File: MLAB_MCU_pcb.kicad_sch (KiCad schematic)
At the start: 0 parts

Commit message: Collecting components and starting work on schematic
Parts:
- added C1, C2, C3, C4: 1u, Capacitor_SMD:C_0805_2012Metric_Pad1.18x1.45mm_HandSolder, symbol Device:C
- added J1, J2: Conn_01x02_Pin, Connector_PinHeader_2.54mm:PinHeader_1x02_P2.54mm_Vertical, symbol Connector:Conn_01x02_Pin
- added J3: Input Header, Connector_PinHeader_2.54mm:PinHeader_1x02_P2.54mm_Vertical, symbol Connector:Conn_01x02_Pin
- added J4: TBC05-02-1-G-G, TerminalBlock_Phoenix:TerminalBlock_Phoenix_MPT-0,5-2-2.54_1x02_P2.54mm_Horizontal, symbol Connector:Screw_Terminal_01x02
- added U1: TPS7A2012PDBVRG4, Package_TO_SOT_SMD:SOT-23-5, symbol Regulator_Linear:TPS7A20xxxDBV
- added U2: TPS7A2033PDBVR, Package_TO_SOT_SMD:SOT-23-5, symbol Regulator_Linear:TPS7A20xxxDBV
- added U3: DSC1101DL5-020.0000, 1_mlab_mcu_fp:VDFN6_2P5X2_MCH, symbol 1_mlab_mcu:DSC1101DL5-020.0000
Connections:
- new net: C2.1, J1.2 (Pin_2), U1.5 (OUT)
- new net: C1.1, J3.1 (Pin_1), J4.2 (Pin_2), U1.1 (IN), U1.3 (EN)
- new net: C3.1, J3.2 (Pin_2), J4.1 (Pin_1), U2.1 (IN), U2.3 (EN)
- new net: C4.1, J2.2 (Pin_2), U2.5 (OUT)
- new net 0: C1.2, C2.2, C3.2, C4.2, U1.2 (GND), U2.2 (GND)

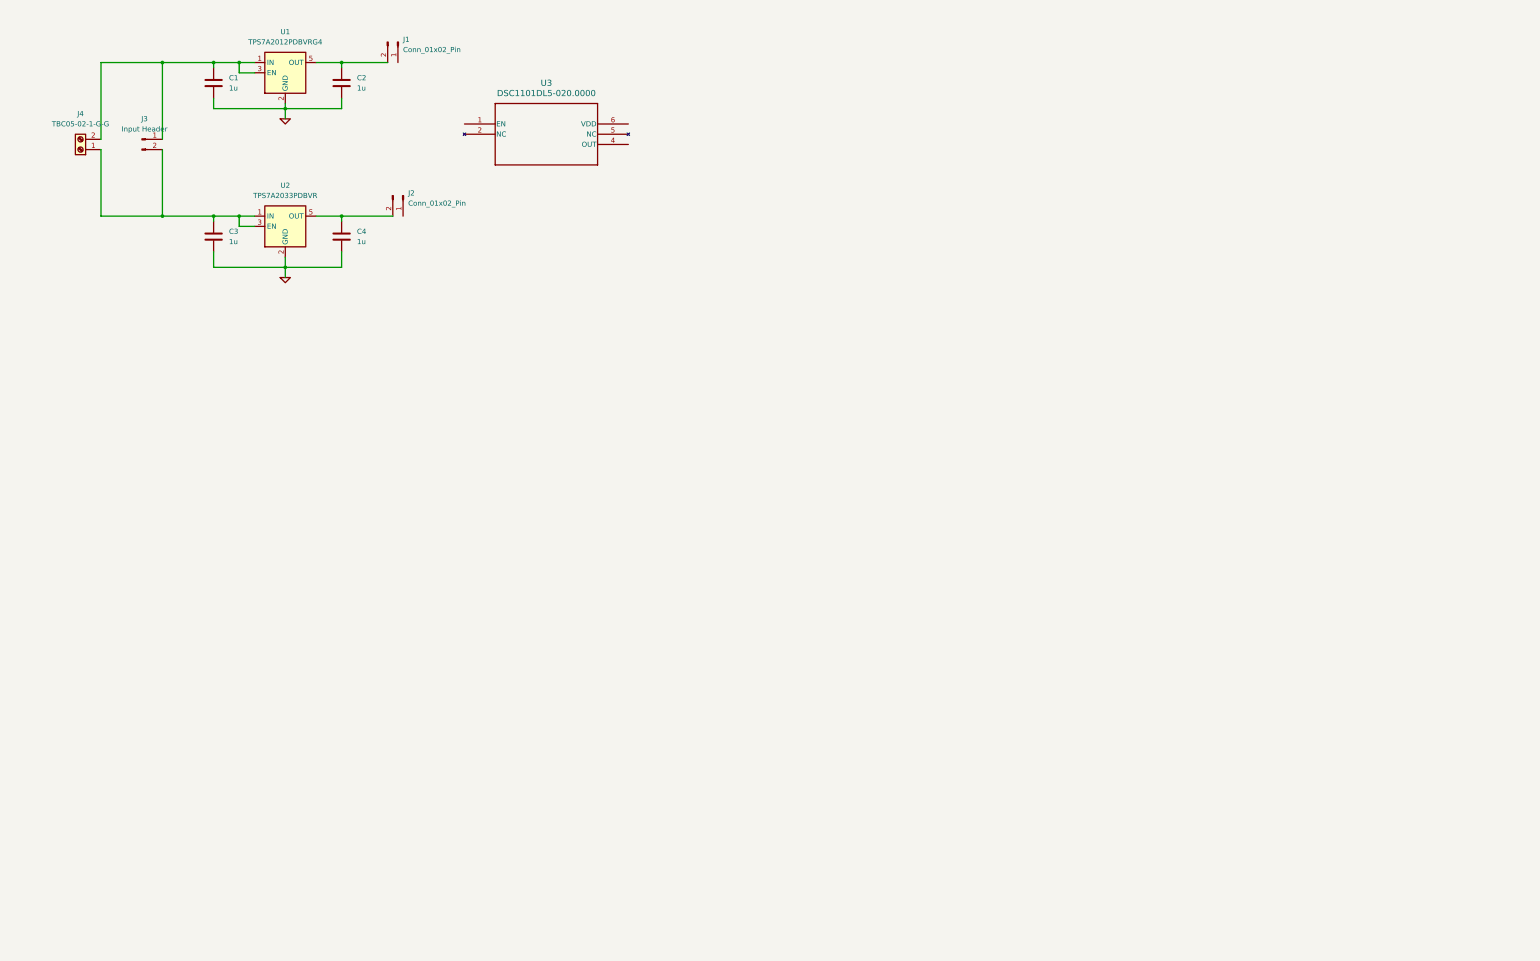
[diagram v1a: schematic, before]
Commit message: Schematic WIP
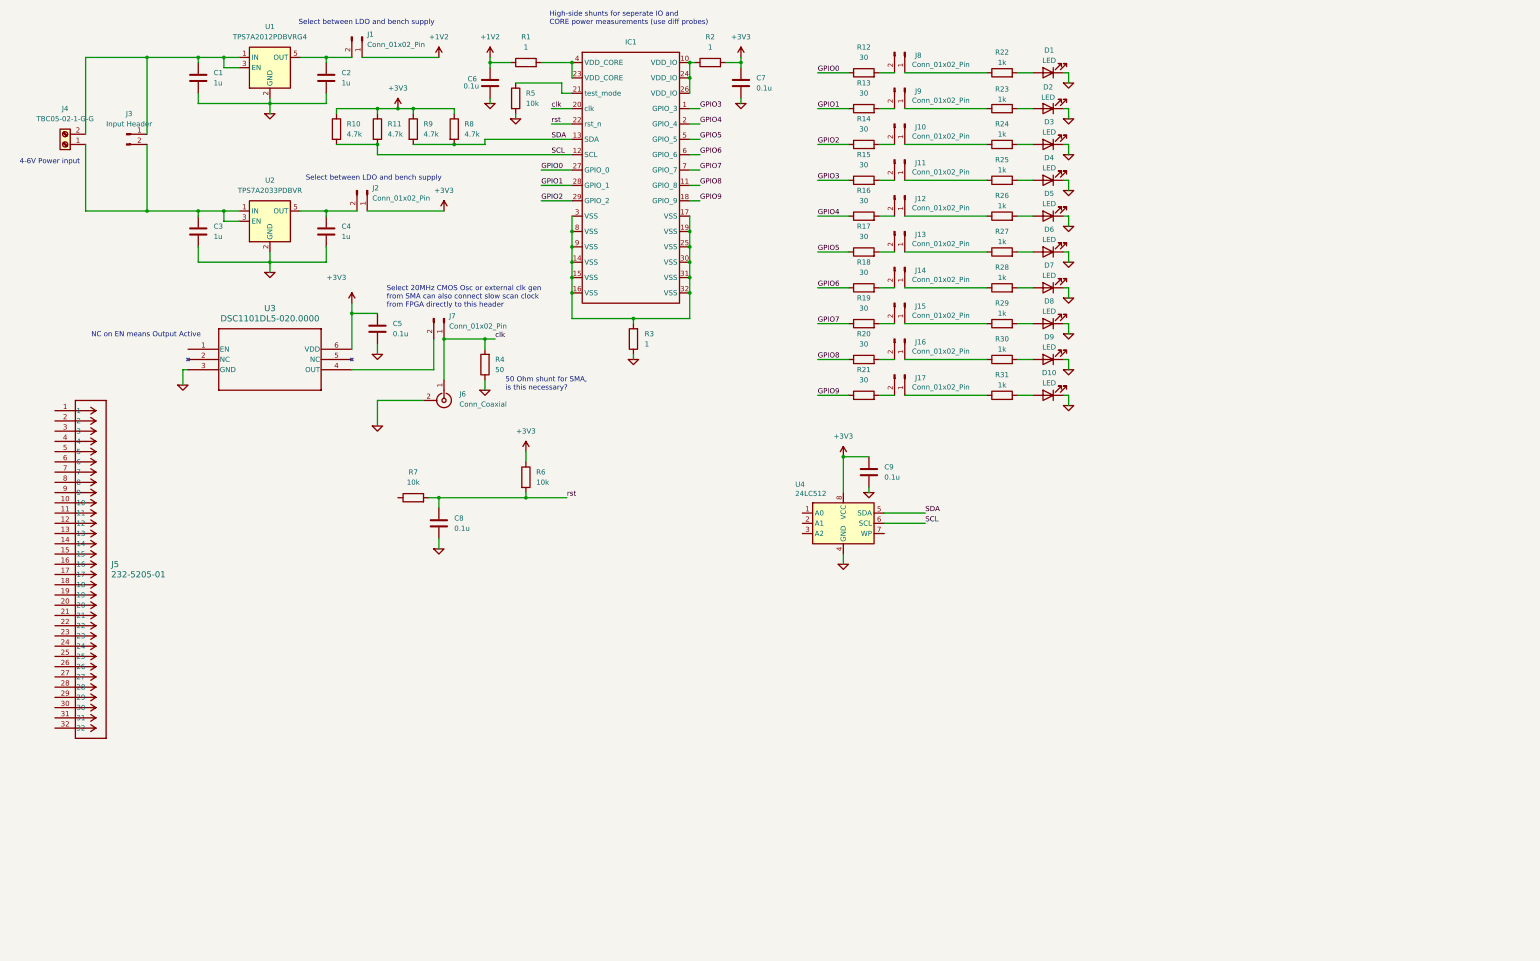
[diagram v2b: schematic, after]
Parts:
- added C5, C6, C7, C8, C9: 0.1u, Capacitor_SMD:C_0805_2012Metric_Pad1.18x1.45mm_HandSolder, symbol Device:C
- added D1, D10, D2, D3, D4, D5, D6, D7, D8, D9: LED, LED_SMD:LED_0805_2012Metric_Pad1.15x1.40mm_HandSolder, symbol Device:LED
- added IC1: (no value), 1_mlab_mcu_fp:VQFN-32-1EP_5x5mm_P0.5mm_EP3.5x3.5mm, symbol 1_mlab_mcu:mlab_mcu
- added J10, J11, J12, J13, J14, J15, J16, J17, J7, J8, J9: Conn_01x02_Pin, Connector_PinHeader_2.54mm:PinHeader_1x02_P2.54mm_Vertical, symbol Connector:Conn_01x02_Pin
- added J5: 232-5205-01, 1_mlab_mcu_fp:CONN_232-5205-01_3MM, symbol 1_mlab_mcu:232-5205-01
- added J6: Conn_Coaxial, Connector_Coaxial:SMA_Amphenol_132134_Vertical, symbol Connector:Conn_Coaxial
- added R1, R2, R3: 1, Resistor_SMD:R_0805_2012Metric_Pad1.20x1.40mm_HandSolder, symbol Device:R
- added R10, R11, R8, R9: 4.7k, Resistor_SMD:R_0805_2012Metric_Pad1.20x1.40mm_HandSolder, symbol Device:R
- added R12, R13, R14, R15, R16, R17, R18, R19, R20, R21: 30, Resistor_SMD:R_0805_2012Metric_Pad1.20x1.40mm_HandSolder, symbol Device:R
- added R22, R23, R24, R25, R26, R27, R28, R29, R30, R31: 1k, Resistor_SMD:R_0805_2012Metric_Pad1.20x1.40mm_HandSolder, symbol Device:R
- added R4: 50, Resistor_SMD:R_0805_2012Metric_Pad1.20x1.40mm_HandSolder, symbol Device:R
- added R5, R6, R7: 10k, Resistor_SMD:R_0805_2012Metric_Pad1.20x1.40mm_HandSolder, symbol Device:R
- added U4: 24LC512, Package_DIP:DIP-8_W7.62mm_Socket, symbol Memory_EEPROM:24LC512
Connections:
- net 0: now also U3.3 (GND), C5.2, C6.2, C7.2, C8.2, C9.2, D1.1 (K), D10.1 (K), D2.1 (K), D3.1 (K), D4.1 (K), D5.1 (K), D6.1 (K), D7.1 (K), D8.1 (K), D9.1 (K), J6.2 (Ext), R3.1, R4.1, R5.2, U4.4 (GND)
- net at U3.4 (OUT): now also J7.2 (Pin_2)
- net +3V3: now reaches U3.6 (VDD)
- net +3V3: now also J2.1 (Pin_1), C5.1, C7.1, C9.1, R10.1, R11.1, R2.2, R6.1, R8.1, R9.1, U4.8 (VCC)
- net +1V2: now reaches J1.1 (Pin_1)
- net +1V2: now also C6.1, R1.1
- new net: J10.1 (Pin_1), R24.1
- new net: J10.2 (Pin_2), R14.2
- new net: J8.1 (Pin_1), R22.1
- new net: J8.2 (Pin_2), R12.2
- new net: IC1.14 (VSS), IC1.15 (VSS), IC1.16 (VSS), IC1.17 (VSS), IC1.19 (VSS), IC1.25 (VSS), IC1.3 (VSS), IC1.30 (VSS), IC1.31 (VSS), IC1.32 (VSS), IC1.8 (VSS), IC1.9 (VSS), R3.2
- new net: J11.1 (Pin_1), R25.1
- new net: D4.2 (A), R25.2
- new net: J15.2 (Pin_2), R19.2
- new net: D3.2 (A), R24.2
- new net: J9.1 (Pin_1), R23.1
- new net: J9.2 (Pin_2), R13.2
- new net: D5.2 (A), R26.2
- new net: J16.2 (Pin_2), R20.2
- new net: D9.2 (A), R30.2
- new net: D8.2 (A), R29.2
- new net: J11.2 (Pin_2), R15.2
- new net: IC1.23 (VDD_CORE), IC1.4 (VDD_CORE), R1.2
- new net: J12.1 (Pin_1), R26.1
- new net: J12.2 (Pin_2), R16.2
- new net: J16.1 (Pin_1), R30.1
- new net: J15.1 (Pin_1), R29.1
- new net: D7.2 (A), R28.2
- new net: IC1.21 (test_mode), R5.1
- new net: J14.1 (Pin_1), R28.1
- new net: J14.2 (Pin_2), R18.2
- new net: D1.2 (A), R22.2
- new net: J17.1 (Pin_1), R31.1
- new net: J17.2 (Pin_2), R21.2
- new net: D2.2 (A), R23.2
- new net: IC1.10 (VDD_IO), IC1.24 (VDD_IO), IC1.26 (VDD_IO), R2.1
- new net: D6.2 (A), R27.2
- new net: J13.2 (Pin_2), R17.2
- new net: D10.2 (A), R31.2
- new net: J13.1 (Pin_1), R27.1
- new net GPIO0: IC1.27 (GPIO_0), R12.1
- new net GPIO1: IC1.28 (GPIO_1), R13.1
- new net GPIO2: IC1.29 (GPIO_2), R14.1
- new net GPIO3: IC1.1 (GPIO_3), R15.1
- new net GPIO4: IC1.2 (GPIO_4), R16.1
- new net GPIO5: IC1.5 (GPIO_5), R17.1
- new net GPIO6: IC1.6 (GPIO_6), R18.1
- new net GPIO7: IC1.7 (GPIO_7), R19.1
- new net GPIO8: IC1.11 (GPIO_8), R20.1
- new net GPIO9: IC1.18 (GPIO_9), R21.1
- new net SCL: IC1.12 (SCL), R10.2, R11.2, U4.6 (SCL)
- new net SDA: IC1.13 (SDA), R8.2, R9.2, U4.5 (SDA)
- new net clk: IC1.20 (clk), J6.1 (In), J7.1 (Pin_1), R4.2
- new net rst: C8.1, IC1.22 (rst_n), R6.2, R7.2
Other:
- note added: "4-6V Power input"
- note added: "50 Ohm shunt for SMA, is this necessary?"
- note added: "High-side shunts for seperate IO and CORE power measurements (use diff probes)"
- note added: "NC on EN means Output Active"
- note added: "Select 20MHz CMOS Osc or external clk gen from SMA can also connect slow scan clock from FPGA directly to this header"
- note added: "Select between LDO and bench supply"
- moved on the sheet: C1, C2, C3, C4, J1, J2, J3, J4, U1, U2

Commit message: Schematic still WIP
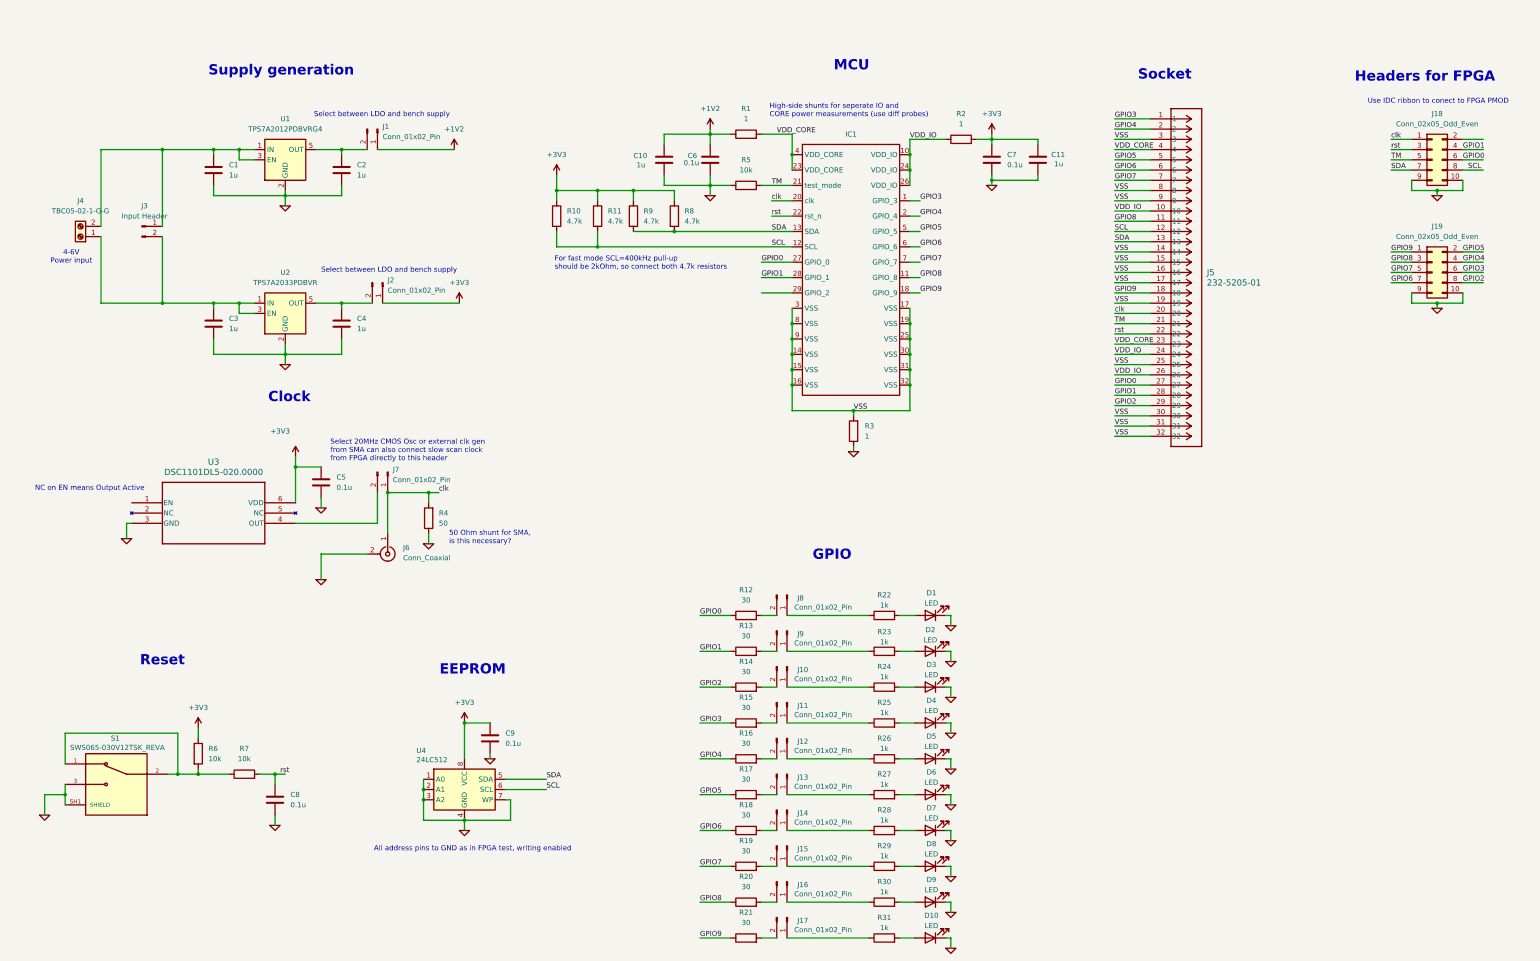
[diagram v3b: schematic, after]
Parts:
- added C10, C11: 1u, Capacitor_SMD:C_0805_2012Metric_Pad1.18x1.45mm_HandSolder, symbol Device:C
- added J18, J19: Conn_02x05_Odd_Even, Connector_PinHeader_2.54mm:PinHeader_2x05_P2.54mm_Vertical, symbol Connector_Generic:Conn_02x05_Odd_Even
- added S1: SWS065-030V12TSK_REVA, 1_mlab_mcu_fp:SW_SWS065-030V12TSK_REVA, symbol 1_mlab_mcu:SWS065-030V12TSK_REVA
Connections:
- net +1V2: now also C10.1
- net +3V3: now also C11.1
- net 0: now also R5.1, U4.1 (A0), U4.2 (A1), U4.3 (A2), U4.7 (WP), C10.2, C11.2, J18.10 (Pin_10), J18.9 (Pin_9), J19.10 (Pin_10), J19.9 (Pin_9), S1.3, S1.SH1 (SHIELD), S1.SH2 (SHIELD); no longer R5.2
- net GPIO0: now also J5.27, J18.6 (Pin_6)
- net GPIO1: now also J5.28, J18.4 (Pin_4)
- net GPIO2: now also J5.29, J19.8 (Pin_8); no longer IC1.29 (GPIO_2)
- net GPIO3: now also J5.1, J19.6 (Pin_6)
- net GPIO4: now also J5.2, J19.4 (Pin_4)
- net GPIO5: now also J5.5, J19.2 (Pin_2)
- net GPIO6: now also J5.6, J19.7 (Pin_7)
- net GPIO7: now also J5.7, J19.5 (Pin_5)
- net GPIO8: now also J5.11, J19.3 (Pin_3)
- net GPIO9: now also J5.18, J19.1 (Pin_1)
- net SCL: now also J5.12, J18.8 (Pin_8)
- net SDA: now also J5.13, J18.7 (Pin_7)
- net clk: now also J5.20, J18.1 (Pin_1)
- net rst: now also J5.22, J18.3 (Pin_3); no longer R6.2
- net VSS: now reaches IC1.14 (VSS), IC1.15 (VSS), IC1.16 (VSS), IC1.17 (VSS), IC1.19 (VSS), IC1.25 (VSS), IC1.3 (VSS), IC1.30 (VSS), IC1.31 (VSS), IC1.32 (VSS), IC1.8 (VSS), IC1.9 (VSS), R3.2
- net VSS: now also J5.14, J5.15, J5.16, J5.17, J5.19, J5.25, J5.3, J5.30, J5.31, J5.32, J5.8, J5.9
- net at R7.1: now also R6.2, S1.1, S1.2
- net VDD_CORE: now reaches IC1.23 (VDD_CORE), IC1.4 (VDD_CORE), R1.2
- net VDD_CORE: now also J5.23, J5.4
- net TM: now reaches IC1.21 (test_mode)
- net TM: now also J5.21, R5.2, J18.5 (Pin_5); no longer R5.1
- net VDD_IO: now reaches IC1.10 (VDD_IO), IC1.24 (VDD_IO), IC1.26 (VDD_IO), R2.1
- net VDD_IO: now also J5.10, J5.24, J5.26
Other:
- note added: "All address pins to GND as in FPGA test, writing enabled"
- note added: "Clock"
- note added: "EEPROM"
- note added: "For fast mode SCL=400kHz pull-up should be 2kOhm, so connect both 4.7k resistors"
- note added: "GPIO"
- note added: "Headers for FPGA"
- note added: "MCU"
- note added: "Reset"
- note added: "Socket"
- note added: "Supply generation"
- note added: "Use IDC ribbon to conect to FPGA PMOD"
- moved on the sheet: C1, C2, C3, C4, C5, C6, C7, C8, C9, D1, D10, D2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
